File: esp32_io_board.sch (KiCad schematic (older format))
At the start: 32 parts

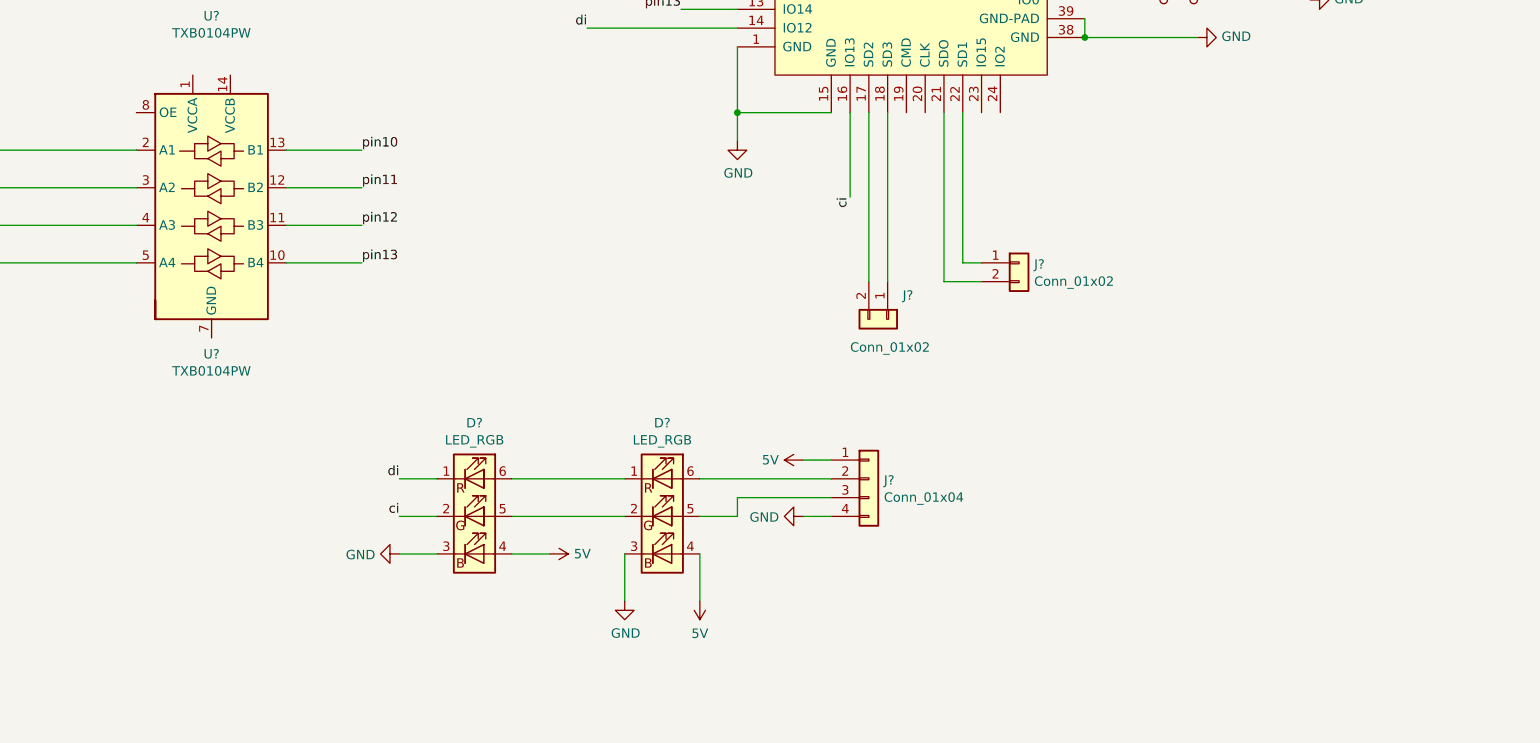
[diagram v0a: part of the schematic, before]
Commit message: tca9548
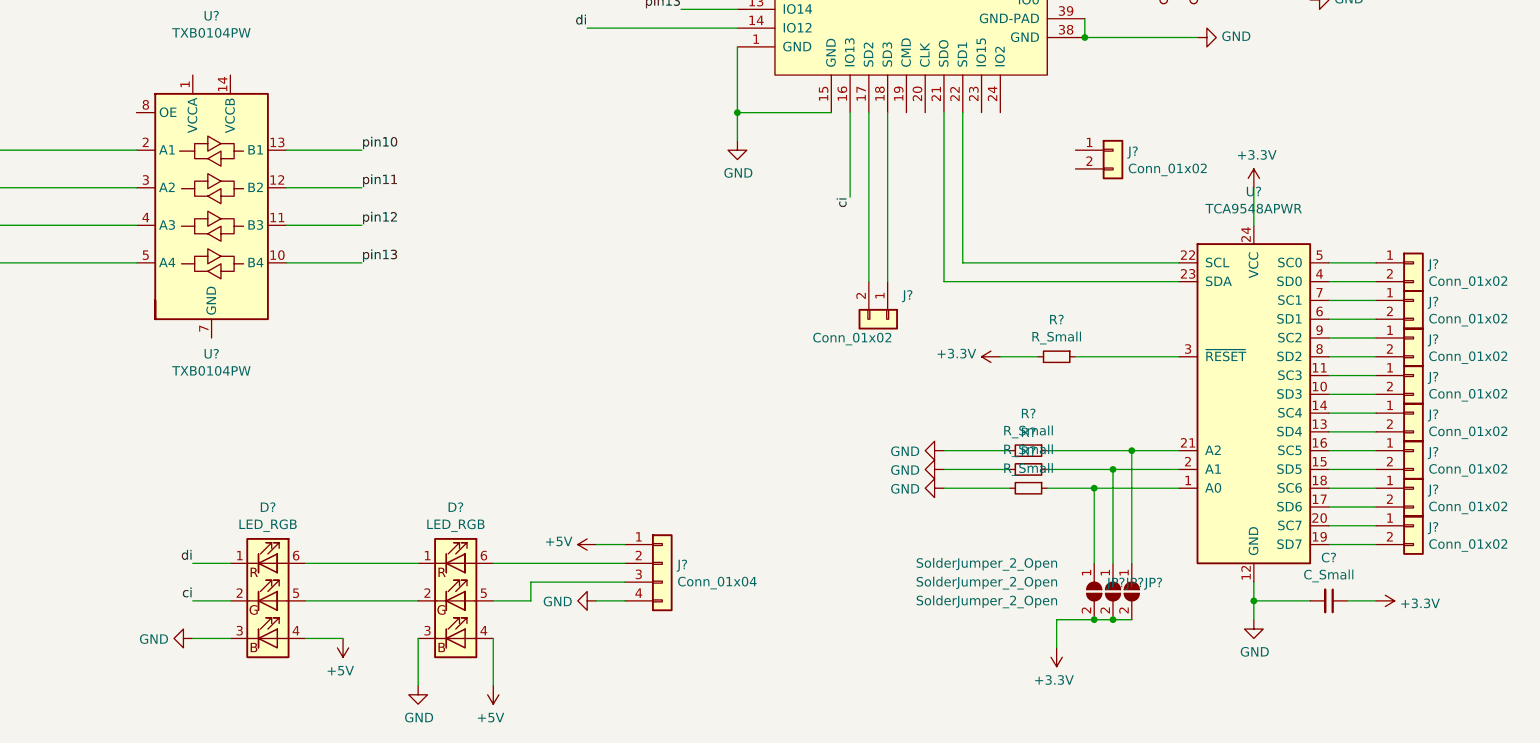
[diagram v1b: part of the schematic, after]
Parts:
- added C?: C_Small, symbol Device:C_Small
- added J? (x8): Conn_01x02, symbol Connector_Generic:Conn_01x02
- added JP? (x3): SolderJumper_2_Open, symbol Jumper:SolderJumper_2_Open
- added R? (x4): R_Small, symbol Device:R_Small
- added U?: TCA9548APWR, Package_SO:TSSOP-24_4.4x7.8mm_P0.65mm, symbol Interface_Expansion:TCA9548APWR
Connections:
- net 5V is gone; now on net +5V: D?.4 (BA), D?.4 (BA), J?.1 (Pin_1)
- net +3V3: now also C?.1, JP?.2 (B), JP?.2 (B), JP?.2 (B), R?.2, U?.24 (VCC)
- net GND: now also C?.2, R?.2, R?.2, R?.2, U?.12 (GND)
- net at U?.21 (SDO): now also U?.23 (SDA); no longer J?.2 (Pin_2)
- net at U?.22 (SD1): now also U?.22 (SCL); no longer J?.1 (Pin_1)
- new net: JP?.1 (A), R?.1, U?.1 (A0)
- new net: J?.2 (Pin_2), U?.10 (SD3)
- new net: J?.1 (Pin_1), U?.11 (SC3)
- new net: J?.2 (Pin_2), U?.13 (SD4)
- new net: J?.1 (Pin_1), U?.14 (SC4)
- new net: J?.2 (Pin_2), U?.15 (SD5)
- new net: J?.1 (Pin_1), U?.16 (SC5)
- new net: J?.2 (Pin_2), U?.17 (SD6)
- new net: J?.1 (Pin_1), U?.18 (SC6)
- new net: J?.2 (Pin_2), U?.19 (SD7)
- new net: JP?.1 (A), R?.1, U?.2 (A1)
- new net: J?.1 (Pin_1), U?.20 (SC7)
- new net: JP?.1 (A), R?.1, U?.21 (A2)
- new net: R?.1, U?.3 (~RESET)
- new net: J?.2 (Pin_2), U?.4 (SD0)
- new net: J?.1 (Pin_1), U?.5 (SC0)
- new net: J?.2 (Pin_2), U?.6 (SD1)
- new net: J?.1 (Pin_1), U?.7 (SC1)
- new net: J?.2 (Pin_2), U?.8 (SD2)
- new net: J?.1 (Pin_1), U?.9 (SC2)
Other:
- moved on the sheet: D?, J?
